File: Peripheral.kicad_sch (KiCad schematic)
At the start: 43 parts, among them J10 Conn_01x03, J11 Conn_01x03, J12 Conn_01x03, J13 Conn_01x03, J2 Conn_01x04, J3 Conn_01x06, J4 Conn_01x06, J5 Conn_01x06, J6 Conn_01x07, J9 Conn_01x03

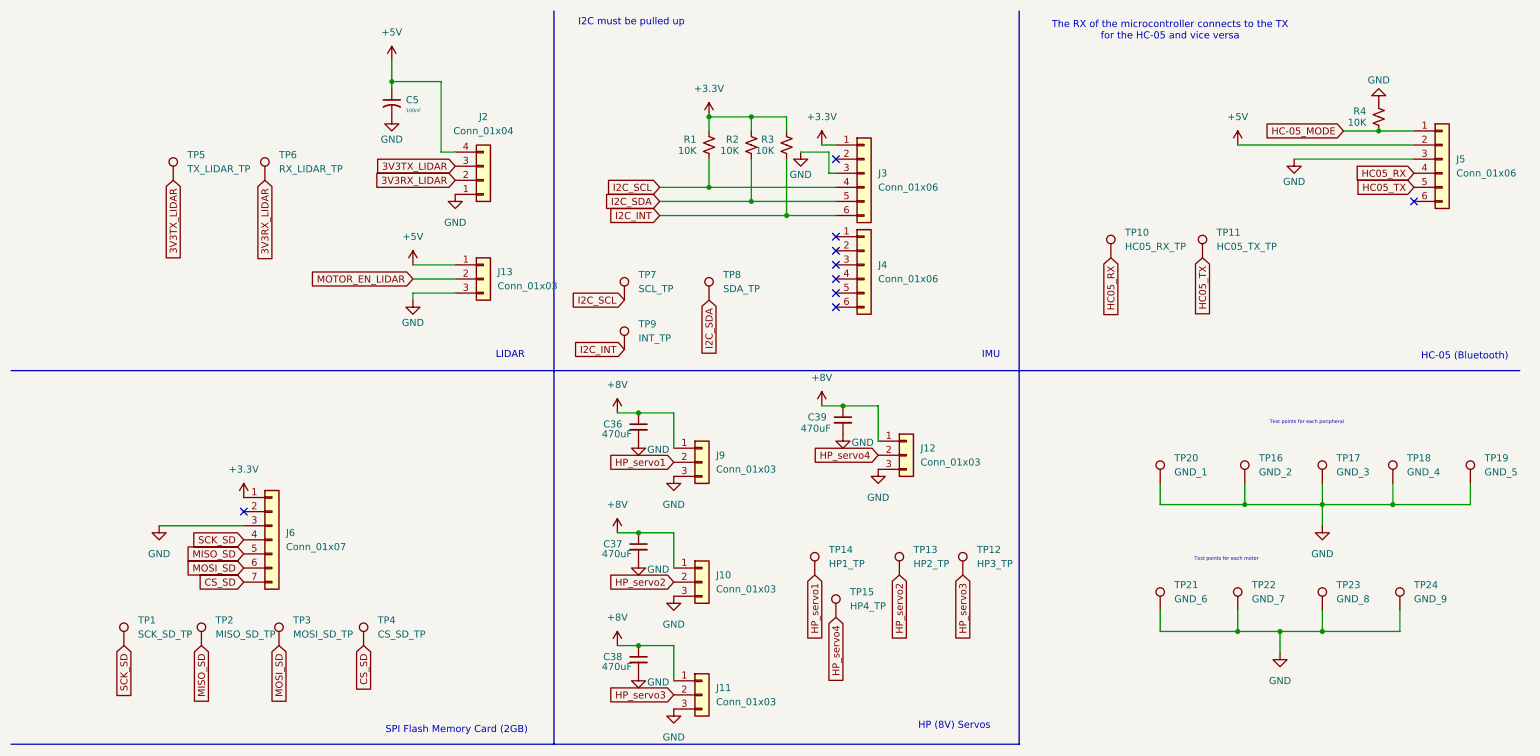
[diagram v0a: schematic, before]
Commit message: almost completed board
need to clean up silkscreen, run thru checklist and verify, review datasheets
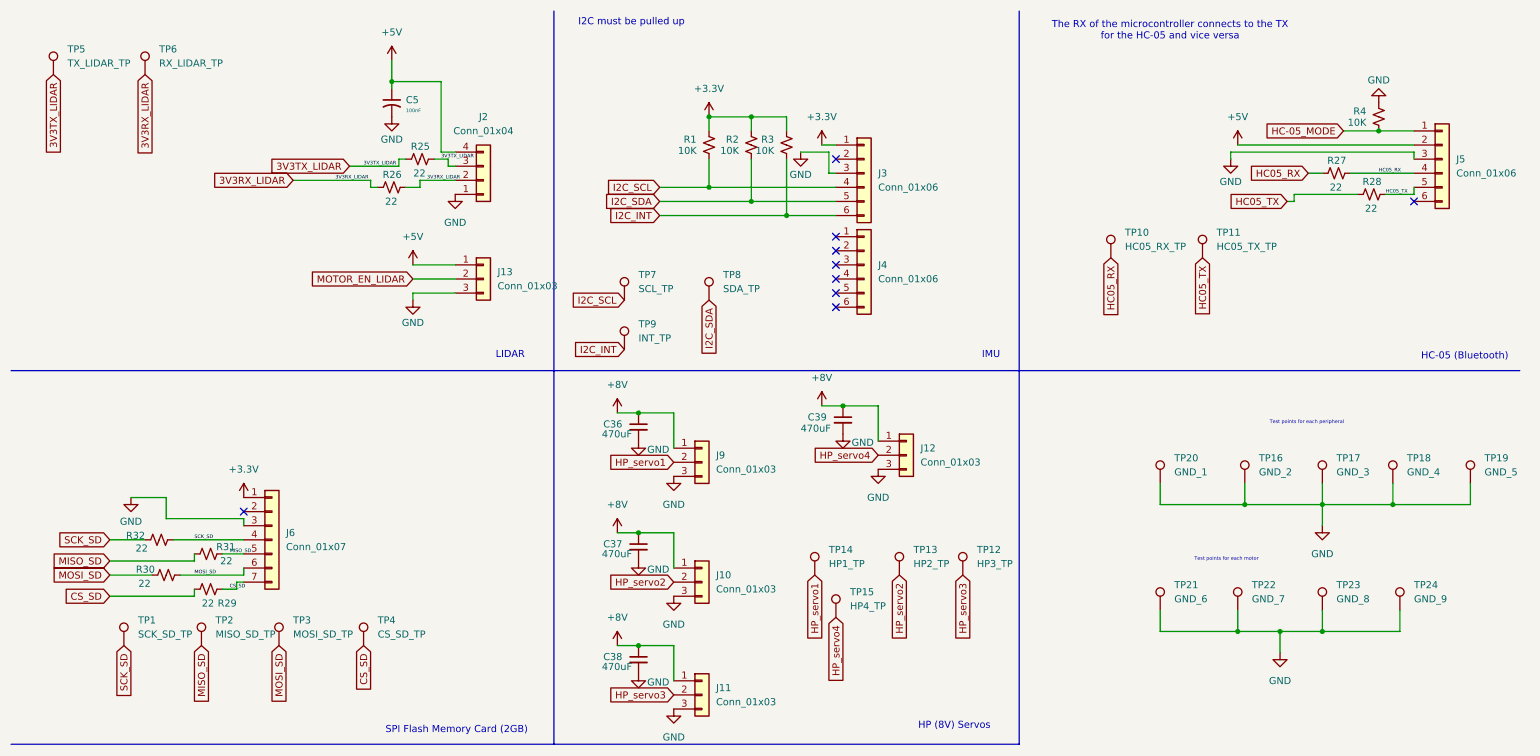
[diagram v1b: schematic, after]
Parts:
- added R25, R26, R27, R28, R29, R30, R31, R32: 22, Resistor_SMD:R_0805_2012Metric_Pad1.20x1.40mm_HandSolder, symbol Device:R_Small_US
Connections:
- net 3V3RX_LIDAR: now also R26.1, R26.2
- net 3V3TX_LIDAR: now also R25.1, R25.2
- net CS_SD: now also R29.1, R29.2
- net HC05_RX: now also R27.1, R27.2
- net HC05_TX: now also R28.1, R28.2
- net MISO_SD: now also R31.1, R31.2
- net MOSI_SD: now also R30.1, R30.2
- net SCK_SD: now also R32.1, R32.2
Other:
- moved on the sheet: TP5, TP6
